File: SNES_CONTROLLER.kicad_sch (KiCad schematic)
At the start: 24 parts, among them J1 Screw_Terminal_01x07, J2 Screw_Terminal_01x12, J3 Screw_Terminal_01x12, U1 4021, U2 4021

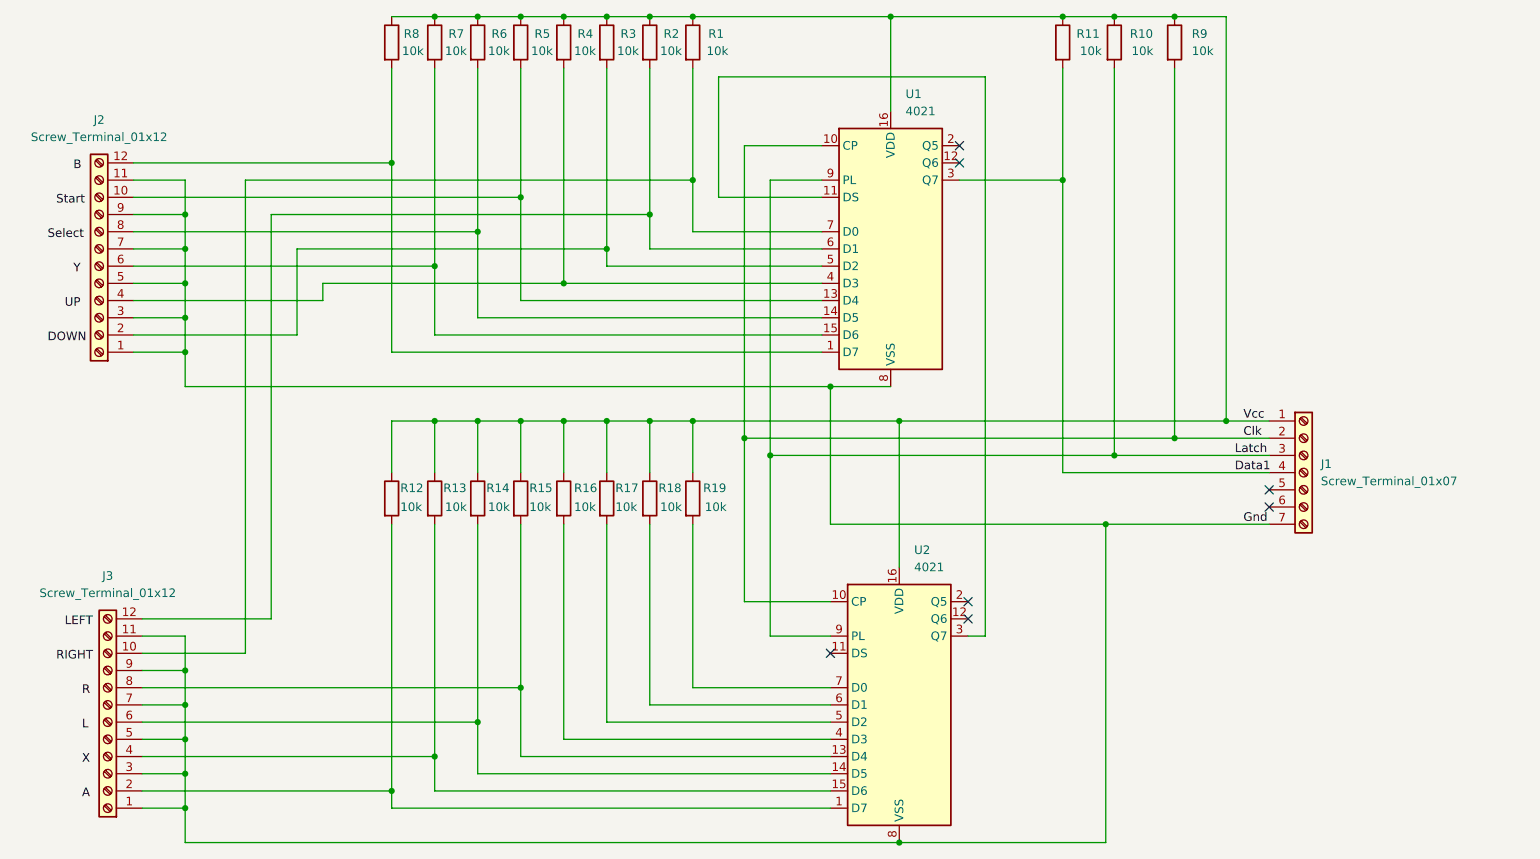
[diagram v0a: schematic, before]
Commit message: SNES CONTROLLER v2
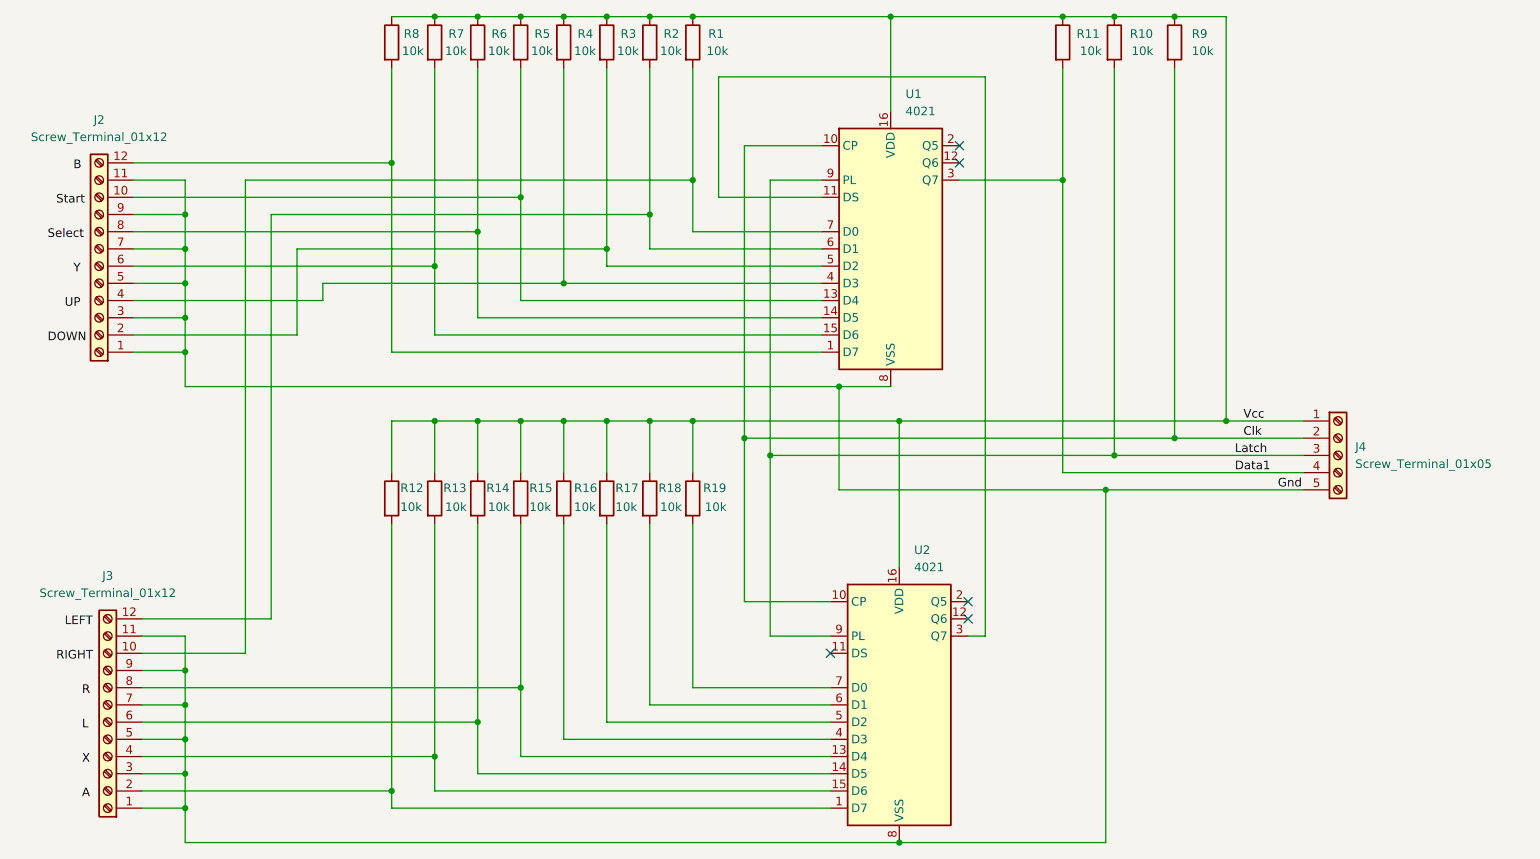
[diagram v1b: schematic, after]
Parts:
- removed J1: Screw_Terminal_01x07, TerminalBlock:TerminalBlock_MaiXu_MX126-5.0-07P_1x07_P5.00mm, symbol Connector:Screw_Terminal_01x07
- added J4: Screw_Terminal_01x05, TerminalBlock:TerminalBlock_MaiXu_MX126-5.0-05P_1x05_P5.00mm, symbol Connector:Screw_Terminal_01x05
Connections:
- net Clk: now also J4.2 (Pin_2)
- net Data1: now also J4.4 (Pin_4)
- net Gnd: now also J4.5 (Pin_5)
- net Latch: now also J4.3 (Pin_3)
- net Vcc: now also J4.1 (Pin_1)
- no-connect marks 7 -> 5
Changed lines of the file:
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@@
+	)
+	(junction
+		(at 142.24 95.25)
+		(diameter 0)
+		(color 0 0 0 0)
 	)
 	(junction
@@
 	)
 	(junction
-		(at 140.97 95.25)
+		(at 181.61 110.49)
 		(diameter 0)
 		(color 0 0 0 0)
@@
 	(junction
 		(at 107.95 40.64)
-		(diameter 0)
-		(color 0 0 0 0)
-	)
-	(junction
-		(at 181.61 115.57)
 		(diameter 0)
 		(color 0 0 0 0)
@@
 	)
 	(no_connect
-		(at 205.74 110.49)
-	)
-	(no_connect
 		(at 161.29 129.54)
 	)
@@
 	)
 	(no_connect
-		(at 205.74 113.03)
-	)
-	(no_connect
 		(at 140.97 134.62)
 	)
@@
 	(wire
 		(pts
-			(xy 205.74 105.41) (xy 182.88 105.41)
+			(xy 182.88 105.41) (xy 210.82 105.41)
 		)
 		(stroke
@@
 	(wire
 		(pts
-			(xy 181.61 115.57) (xy 205.74 115.57)
-		)
-		(stroke
-			(width 0)
-			(type default)
-		)
-	)
-	(wire
-		(pts
 			(xy 45.72 80.01) (xy 45.72 74.93)
 		)
@@
 	(wire
 		(pts
-			(xy 140.97 95.25) (xy 140.97 115.57)
+			(xy 142.24 95.25) (xy 142.24 110.49)
 		)
 		(stroke
@@
 	(wire
 		(pts
-			(xy 205.74 102.87) (xy 191.77 102.87)
+			(xy 191.77 102.87) (xy 210.82 102.87)
 		)
 		(stroke
@@
 	(wire
 		(pts
-			(xy 199.39 100.33) (xy 205.74 100.33)
+			(xy 199.39 100.33) (xy 210.82 100.33)
 		)
 		(stroke
@@
 	(wire
 		(pts
-			(xy 181.61 115.57) (xy 181.61 162.56)
-		)
-		(stroke
-			(width 0)
-			(type default)
-		)
-	)
-	(wire
-		(pts
 			(xy 38.1 67.31) (xy 95.25 67.31)
 		)
@@
 	(wire
 		(pts
-			(xy 140.97 115.57) (xy 181.61 115.57)
+			(xy 142.24 110.49) (xy 181.61 110.49)
 		)
 		(stroke
@@
 	(wire
 		(pts
-			(xy 205.74 107.95) (xy 175.26 107.95)
+			(xy 175.26 107.95) (xy 210.82 107.95)
 		)
 		(stroke
@@
 	(wire
 		(pts
+			(xy 181.61 110.49) (xy 210.82 110.49)
+		)
+		(stroke
+			(width 0)
+			(type default)
+		)
+	)
+	(wire
+		(pts
 			(xy 82.55 149.86) (xy 82.55 154.94)
 		)
@@
 	(wire
 		(pts
-			(xy 45.72 95.25) (xy 140.97 95.25)
+			(xy 45.72 95.25) (xy 142.24 95.25)
 		)
 		(stroke
@@
 	(wire
 		(pts
+			(xy 181.61 110.49) (xy 181.61 162.56)
+		)
+		(stroke
+			(width 0)
+			(type default)
+		)
+	)
+	(wire
+		(pts
 			(xy 107.95 144.78) (xy 107.95 115.57)
 		)
@@
 	(wire
 		(pts
-			(xy 149.86 95.25) (xy 140.97 95.25)
+			(xy 149.86 95.25) (xy 142.24 95.25)
 		)
 		(stroke
@@
 	)
 	(label "Gnd"
-		(at 201.93 115.57 0)
+		(at 207.01 110.49 0)
 		(effects
 			(font
@@
 				(path "/719592b0-85a8-4eb6-8d13-f447981f3475"
 					(reference "R7")
-					(unit 1)
-				)
-			)
-		)
-	)
-	(symbol
-		(lib_id "Connector:Screw_Terminal_01x07")
-		(at 210.82 107.95 0)
-		(unit 1)
-		(exclude_from_sim no)
-		(in_bom yes)
-		(on_board yes)
-		(dnp no)
-		(fields_autoplaced yes)
-		(property "Reference" "J1"
-			(at 213.36 106.6799 0)
-			(effects
-				(font
-					(size 1.27 1.27)
-				)
-				(justify left)
-			)
-		)
-		(property "Value" "Screw_Terminal_01x07"
-			(at 213.36 109.2199 0)
-			(effects
-				(font
-					(size 1.27 1.27)
-				)
-				(justify left)
-			)
-		)
-		(property "Footprint" "TerminalBlock:TerminalBlock_MaiXu_MX126-5.0-07P_1x07_P5.00mm"
-			(at 210.82 107.95 0)
-			(effects
-				(font
-					(size 1.27 1.27)
-				)
-				(hide yes)
-			)
-		)
-		(property "Datasheet" "~"
-			(at 210.82 107.95 0)
-			(effects
-				(font
-					(size 1.27 1.27)
-				)
-				(hide yes)
-			)
-		)
-		(property "Description" "Generic screw terminal, single row, 01x07, script generated (kicad-library-utils/schlib/autogen/connector/)"
-			(at 210.82 107.95 0)
-			(effects
-				(font
-					(size 1.27 1.27)
-				)
-				(hide yes)
-			)
-		)
-		(pin "7"
-		)
-		(pin "6"
-		)
-		(pin "5"
-		)
-		(pin "4"
-		)
-		(pin "2"
-		)
-		(pin "3"
-		)
-		(pin "1"
-		)
-		(instances
-			(project ""
-				(path "/719592b0-85a8-4eb6-8d13-f447981f3475"
-					(reference "J1")
 					(unit 1)
 				)
@@
 					(unit 1)
 				)
+			)
+		)
+	)
+	(symbol
+		(lib_id "Connector:Screw_Terminal_01x05")
+		(at 215.9 105.41 0)
+		(unit 1)
+		(exclude_from_sim no)
+		(in_bom yes)
+		(on_board yes)
+		(dnp no)
+		(fields_autoplaced yes)
+		(property "Reference" "J4"
+			(at 218.44 104.1399 0)
+			(effects
+				(font
+					(size 1.27 1.27)
+				)
+				(justify left)
+			)
+		)
+		(property "Value" "Screw_Terminal_01x05"
+			(at 218.44 106.6799 0)
+			(effects
+				(font
+					(size 1.27 1.27)
+				)
+				(justify left)
+			)
+		)
+		(property "Footprint" "TerminalBlock:TerminalBlock_MaiXu_MX126-5.0-05P_1x05_P5.00mm"
+			(at 215.9 105.41 0)
+			(effects
+				(font
+					(size 1.27 1.27)
+				)
+				(hide yes)
+			)
+		)
+		(property "Datasheet" "~"
+			(at 215.9 105.41 0)
+			(effects
+				(font
+					(size 1.27 1.27)
+				)
+				(hide yes)
+			)
+		)
+		(property "Description" "Generic screw terminal, single row, 01x05, script generated (kicad-library-utils/schlib/autogen/connector/)"
+			(at 215.9 105.41 0)
+			(effects
+				(font
+					(size 1.27 1.27)
+				)
+				(hide yes)
+			)
+		)
+		(pin "5"
+		)
+		(pin "1"
+		)
+		(pin "4"
+		)
+		(pin "3"
+		)
+		(pin "2"
+		)
+		(instances
+			(project ""
+				(path "/719592b0-85a8-4eb6-8d13-f447981f3475"
+					(reference "J4")
+					(unit 1)
+				)
